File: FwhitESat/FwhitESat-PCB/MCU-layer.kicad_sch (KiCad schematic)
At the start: 1 part, among them U3 Pico

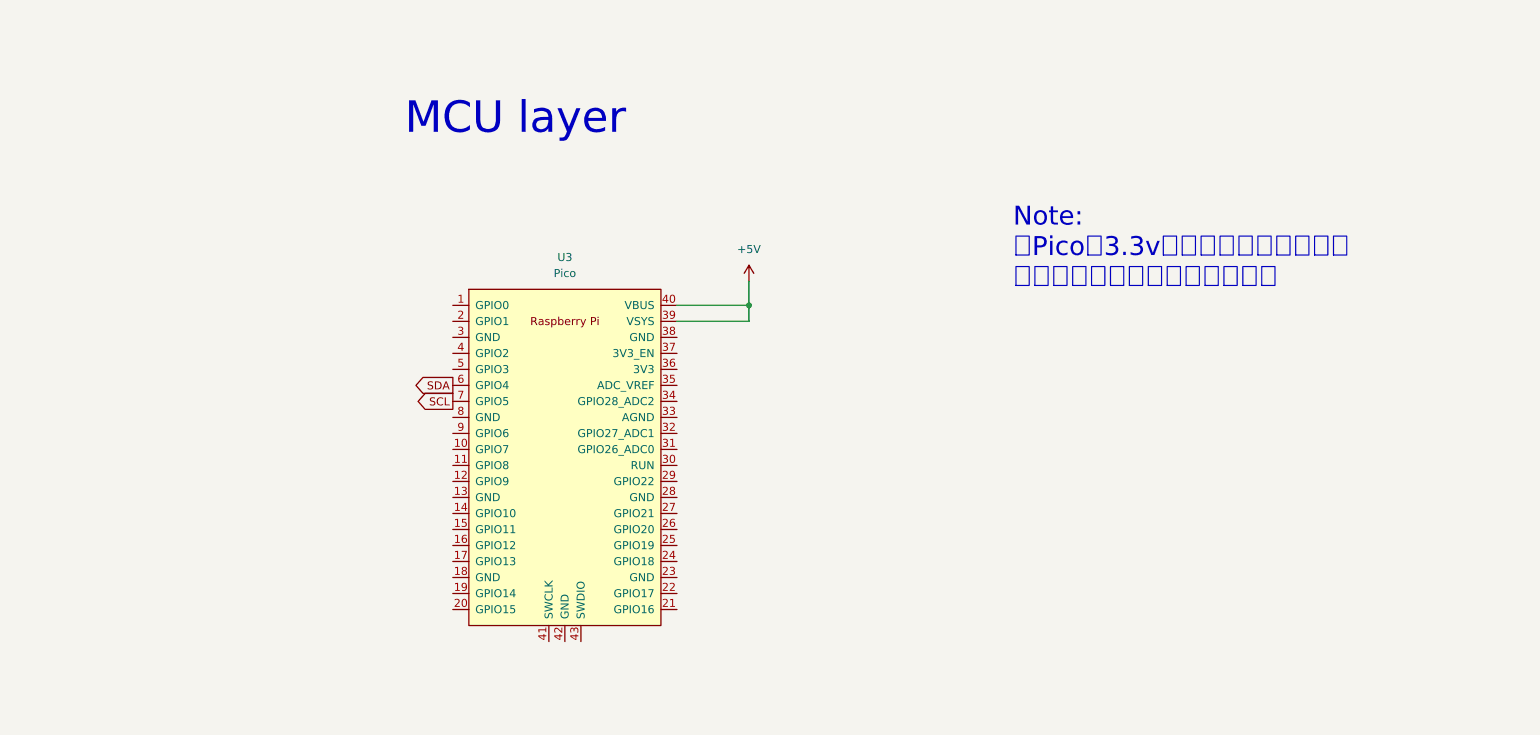
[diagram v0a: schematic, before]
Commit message: くっぱ
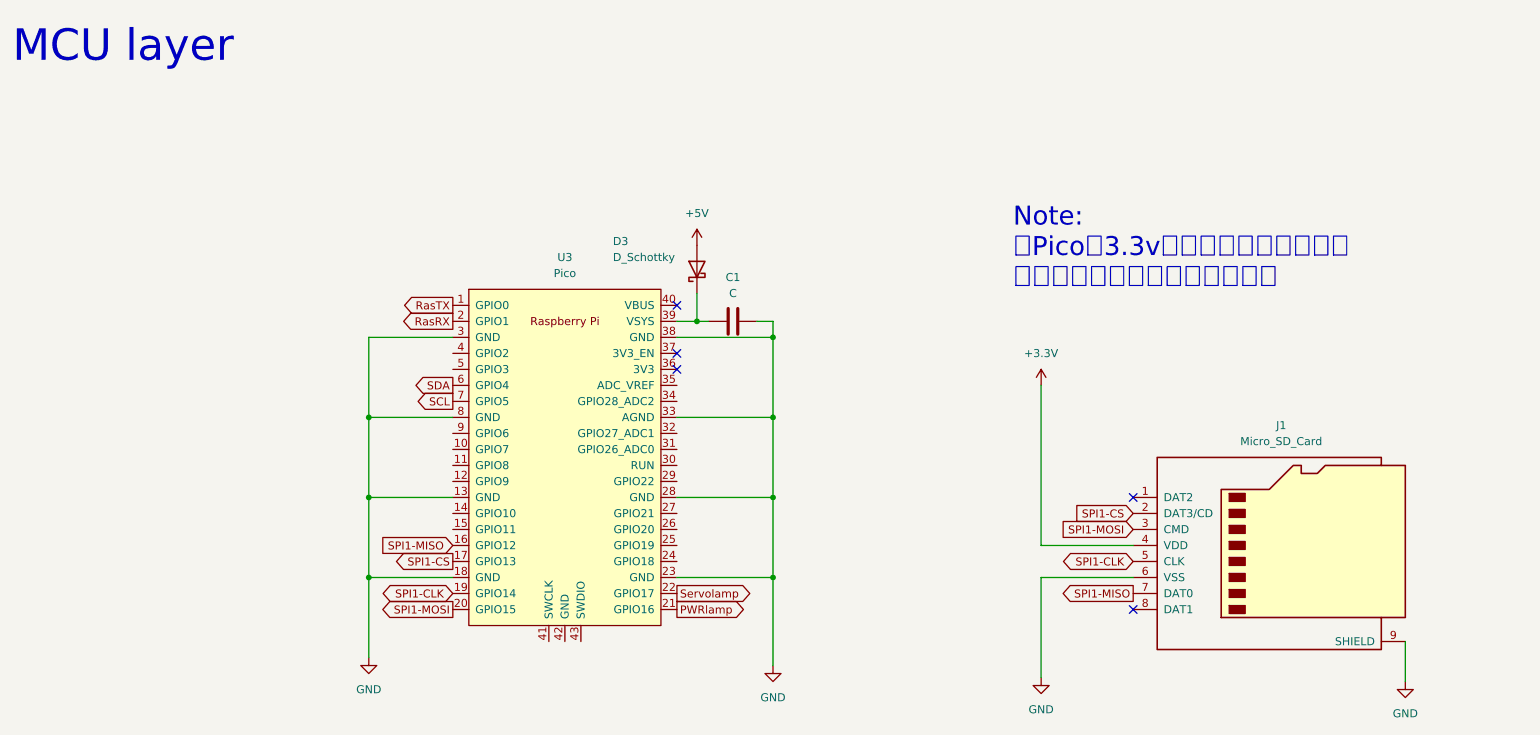
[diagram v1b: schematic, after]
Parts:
- added C1: C, symbol 01-FwhitESat-Local_Library:C
- added D3: D_Schottky, symbol 01-FwhitESat-Local_Library:D_Schottky
- added J1: Micro_SD_Card, symbol 01-FwhitESat-Local_Library:Micro_SD_Card
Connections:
- net +5V: now also D3.2 (A); no longer U3.39 (VSYS), U3.40 (VBUS)
- net RasTX: now reaches U3.1 (GPIO0)
- net GND: now reaches U3.13 (GND)
- net GND: now also U3.18 (GND), U3.23 (GND), U3.28 (GND), U3.3 (GND), U3.33 (AGND), U3.38 (GND), U3.8 (GND), C1.2, J1.6 (VSS), J1.9 (SHIELD)
- net SPI1-MISO: now reaches U3.16 (GPIO12)
- net SPI1-MISO: now also J1.7 (DAT0)
- net SPI1-CS: now reaches U3.17 (GPIO13)
- net SPI1-CS: now also J1.2 (DAT3/CD)
- net SPI1-CLK: now reaches U3.19 (GPIO14)
- net SPI1-CLK: now also J1.5 (CLK)
- net RasRX: now reaches U3.2 (GPIO1)
- net SPI1-MOSI: now reaches U3.20 (GPIO15)
- net SPI1-MOSI: now also J1.3 (CMD)
- net PWRlamp: now reaches U3.21 (GPIO16)
- net Servolamp: now reaches U3.22 (GPIO17)
- new net: C1.1, D3.1 (K), U3.39 (VSYS)
- new net +3.3V: J1.4 (VDD)
- no-connect marks 0 -> 5
